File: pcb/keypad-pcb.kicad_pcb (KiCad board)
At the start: 2 copper layers, 38.1 x 59.9 mm, 20 parts, among them SW1 SW_Push, U1 ATmega32U4-A, Y1 Crystal_GND24_Small

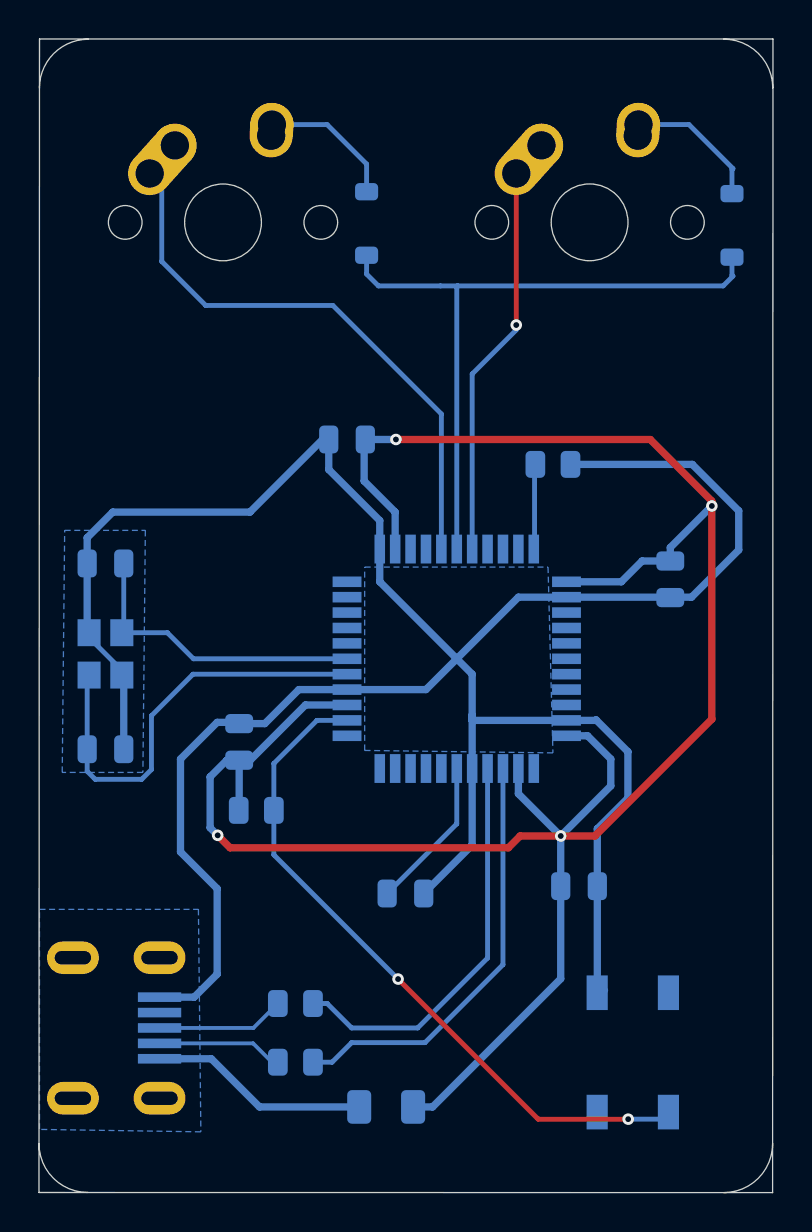
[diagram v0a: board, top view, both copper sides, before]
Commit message: finalized pcb and created gerbers
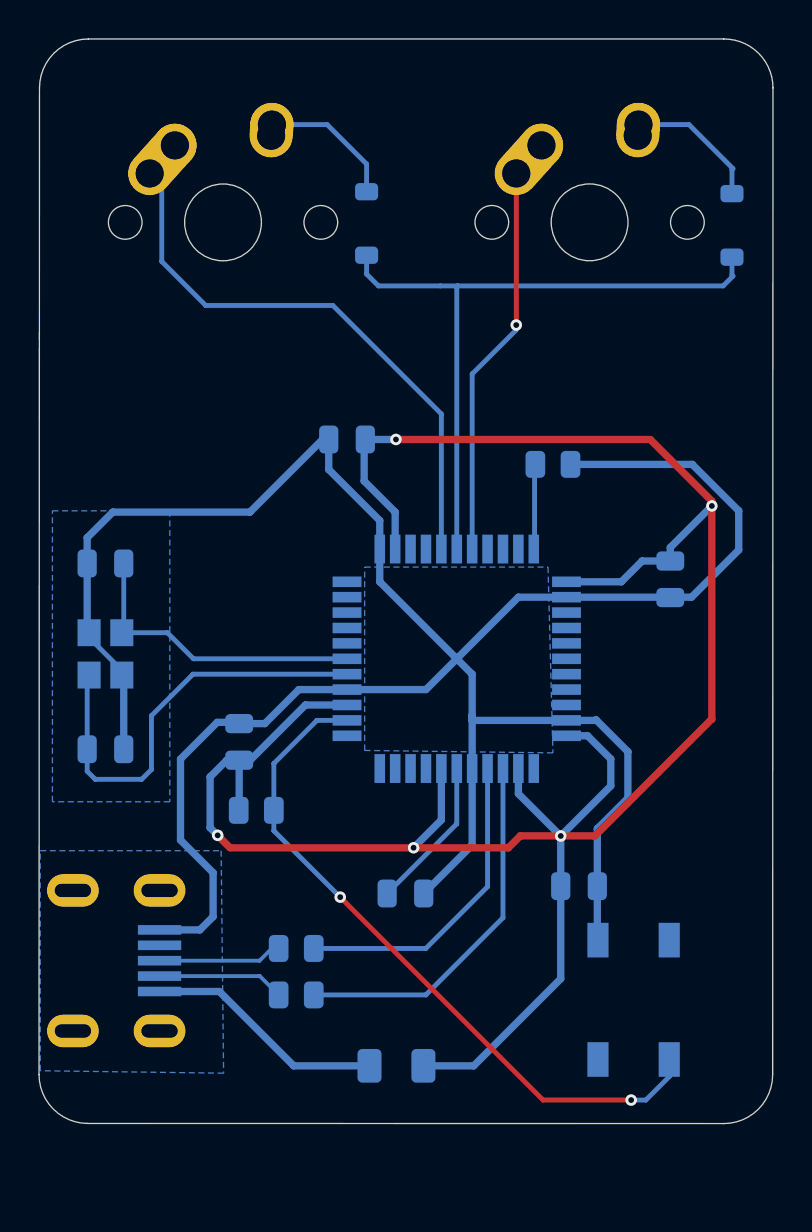
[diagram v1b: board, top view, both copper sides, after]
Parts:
- moved R3 3.49 mm to (71.1, 88.4)
- moved USB1 3.49 mm to (59.5, 86.6)
- moved R2 2.86 mm to (71.1, 86.0)
- moved SW1 2.73 mm to (88.6, 88.6)
- moved F1 2.20 mm to (76.3, 92.1)
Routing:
- net GND: track 137.9 -> 131.7 mm
- net Net-(U1-D+): track 20.9 -> 16.5 mm
- net +5V: track 119.9 -> 123.2 mm, vias 4 -> 5
- net Net-(U1-D-): track 22.2 -> 19.2 mm
- net VCC: track 11.4 -> 12.5 mm
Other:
- board size 38.1 x 59.9 mm -> 38.1 x 56.3 mm
